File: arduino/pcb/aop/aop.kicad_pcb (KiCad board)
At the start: 2 copper layers, 45 x 60 mm, 13 parts, among them J1 Conn_01x02_Pin, M1 RFID-RC522, Q1 AO4435, SW1 SW_Push, U1 ESP32-C3_SUPERMINI_TH, U2 TC00500

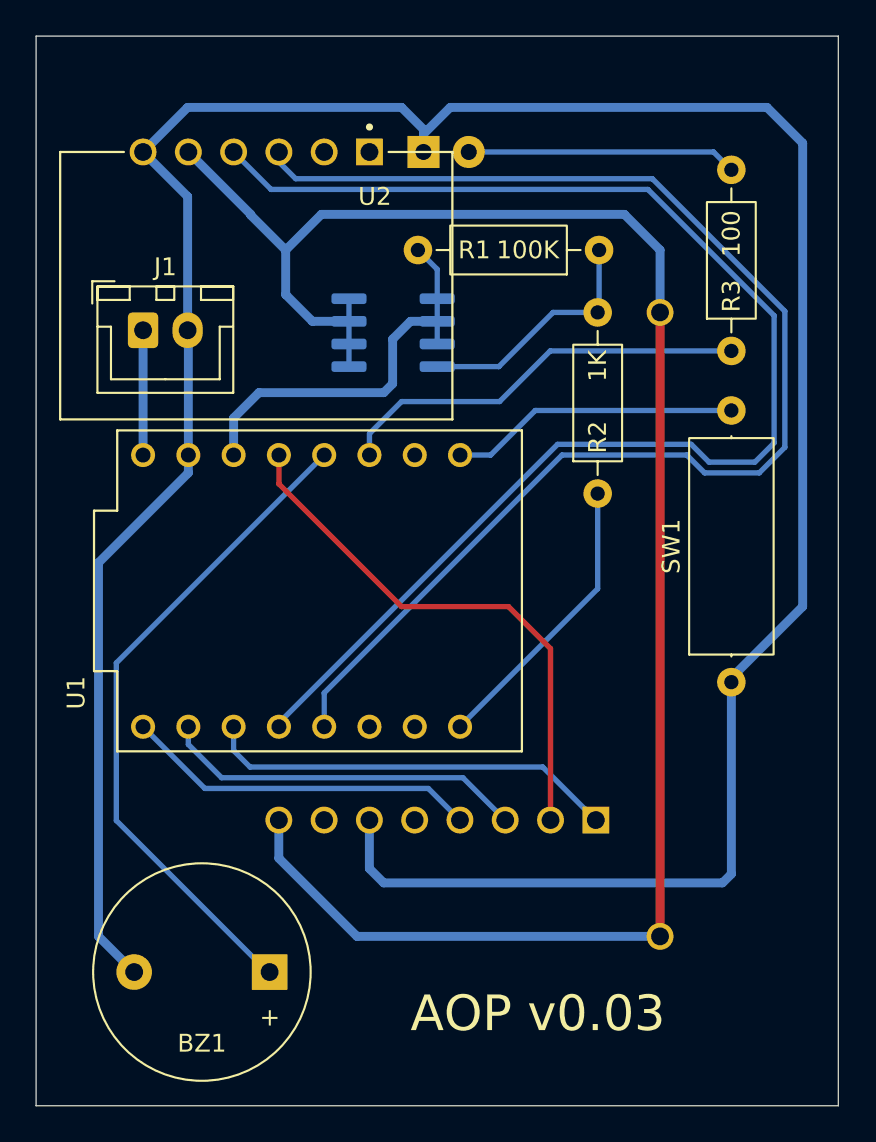
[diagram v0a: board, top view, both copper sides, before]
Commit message: [pcb] AOP v0.1
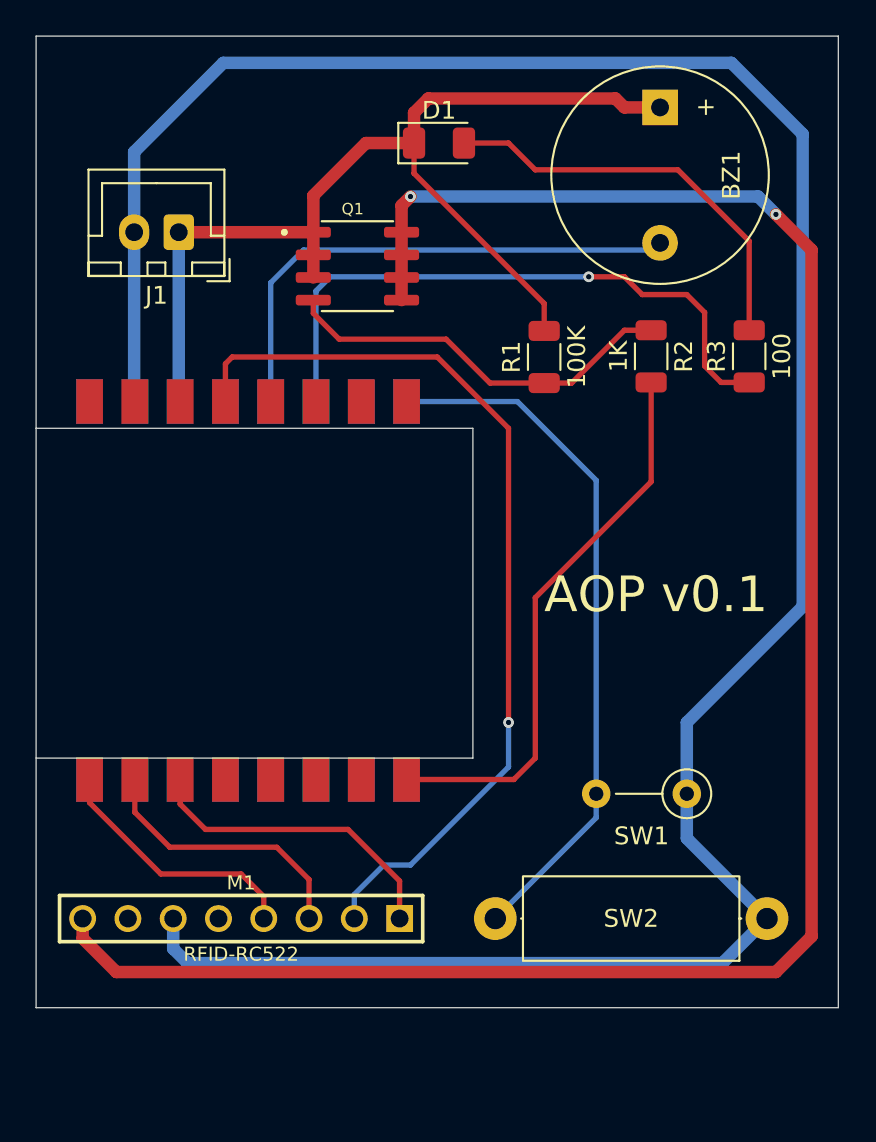
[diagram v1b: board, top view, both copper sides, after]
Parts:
- removed the ? at (104.5, 89.0)
- removed the ? at (104.5, 124.0)
- removed U1: ESP32-C3_SUPERMINI_TH, ESP32-C3_SUPERMINI_TH:MODULE_ESP32-C3_SUPERMINI_TH
- removed U2: TC00500, TC00500:MODULE_TC00500
- added ?: , , F.Cu at (80.0, 94.0)
- added ?: , , F.Cu at (82.5, 115.0)
- added ?: , , F.Cu at (75.0, 94.0)
- added ?: , , F.Cu at (82.5, 94.0)
- added ?: , , F.Cu at (87.5, 115.0)
- added ?: , , F.Cu at (87.5, 94.0)
- added ?: , , F.Cu at (75.0, 115.0)
- added ?: , , F.Cu at (90.0, 115.0)
- added ?: , , B.Cu at (72.5, 115.5)
- added ?: , , B.Cu at (90.0, 115.5)
- added ?: , , B.Cu at (75.0, 94.0)
- added ?: , , F.Cu at (90.0, 94.0)
- added ?: , , B.Cu at (72.5, 94.0)
- added ?: , , B.Cu at (75.0, 115.5)
- added ?: , , B.Cu at (90.5, 94.0)
- added ?: , , B.Cu at (77.5, 115.5)
- added ?: , , B.Cu at (82.5, 115.5)
- added ?: , , B.Cu at (80.0, 94.0)
- added ?: , , B.Cu at (77.5, 94.0)
- added ?: , , B.Cu at (80.0, 115.5)
- added ?: , , B.Cu at (87.5, 115.5)
- added ?: , , B.Cu at (88.0, 94.0)
- added ?: , , F.Cu at (77.5, 94.0)
- added ?: , , B.Cu at (85.0, 115.5)
- added ?: , , B.Cu at (82.5, 94.0)
- added ?: , , B.Cu at (85.0, 94.0)
- added ?: , , F.Cu at (77.5, 115.0)
- added ?: , , F.Cu at (72.5, 94.0)
- added ?: , , F.Cu at (85.0, 115.0)
- added ?: , , F.Cu at (85.0, 94.0)
- added ?: , , F.Cu at (72.5, 115.0)
- added ?: , , F.Cu at (80.0, 115.0)
- added SW2: SW_Push, Resistor_THT:R_Axial_DIN0414_L11.9mm_D4.5mm_P15.24mm_Horizontal, F.Cu at (110.5, 123.0)
- D1: footprint LED_THT:LED_D3.0mm -> LED_SMD:LED_1206_3216Metric; moved to F.Cu
- M1: footprint RFID-RC522:RFID-RC522 -> RFID-RC522:RFID-RC522_1; moved to F.Cu
- Q1: moved to F.Cu
- R1, R2, R3: footprint Resistor_THT:R_Axial_DIN0207_L6.3mm_D2.5mm_P10.16mm_Horizontal -> Resistor_SMD:R_1206_3216Metric
- SW1: footprint Resistor_THT:R_Axial_DIN0414_L11.9mm_D4.5mm_P15.24mm_Horizontal -> Resistor_THT:R_Axial_DIN0207_L6.3mm_D2.5mm_P5.08mm_Vertical
- moved BZ1 53.2 mm to (104.5, 77.5), turned to -90 degrees
- moved M1 12.3 mm to (81.0, 123.0)
- moved R2 8.26 mm to (104.0, 91.5), turned to -90 degrees
- moved R1 6.74 mm to (98.0, 91.5), turned to 90 degrees
- moved SW1 6.74 mm to (106.0, 116.0), turned to 180 degrees
- moved J1 5.85 mm to (77.5, 84.5), turned to 180 degrees
- moved Q1 4.23 mm to (87.5, 86.4), turned to 0 degrees
- moved R3 1.04 mm to (109.5, 91.5)
- moved D1 1.00 mm to (92.1, 79.5)
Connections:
- BZ1 pad 1: Net-(BZ1-+) -> +BATT
- BZ1 pad 2: GND -> Net-(BZ1--)
- D1 pad 1: GND -> +BATT
- Q1 pad 1: Net-(U1-3V3) -> +BATT
- Q1 pad 2: Net-(U1-3V3) -> +BATT
- Q1 pad 3: Net-(U1-3V3) -> +BATT
- R1 pad 2: Net-(U1-3V3) -> +BATT
- R2 pad 1: Net-(U1-GPIO21) -> Net-(Q1-Pad4)
- R2 pad 2: Net-(Q1-Pad4) -> Net-(U1-GPIO21)
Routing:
- net Net-(U1-GPIO8): track 76.6 -> 0.00 mm
- net Net-(U1-GPIO9): track 74.3 -> 0.00 mm
- net +BATT: track 7.00 -> 58.1 mm
- net Net-(BZ1-+): track 37.5 -> 0.00 mm
- net Net-(BZ1--): track 0.00 -> 29.4 mm
- net Net-(U1-GPIO0): track 16.3 -> 39.4 mm
- net Net-(U1-3V3): track 22.9 -> 0.00 mm
- net Net-(M1-SCK): track 30.3 -> 51.8 mm, vias 0 -> 1
- net GND: track 156.9 -> 140.2 mm
- net Net-(U1-GPIO21): track 16.3 -> 31.5 mm
- net Net-(U1-GPIO2): track 23.4 -> 35.0 mm, vias 0 -> 1
- net Net-(D1-A): track 14.4 -> 23.3 mm
- net Net-(Q1-Pad4): track 13.8 -> 22.5 mm
- net +3.3VA: track 104.7 -> 111.9 mm, vias 0 -> 2
- net Net-(M1-SDA): track 23.3 -> 17.6 mm
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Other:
- board size 45 x 60 mm -> 45 x 54.5 mm
- board text added: "AOP v0.1"
- board text removed: "AOP v0.03"
